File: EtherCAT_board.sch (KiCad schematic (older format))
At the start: 28 parts, among them J1 CONN_01X12, J2 USB_OTG, J3 RJ45-PULSETRANS, J4 RJ45-PULSETRANS, SW1 SKRPACE010, U1 LAN9252, U2 LM1117-3.3

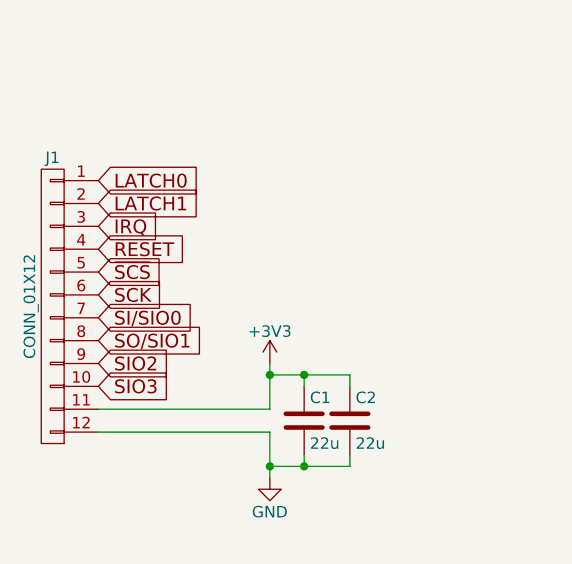
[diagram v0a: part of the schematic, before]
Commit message: 進捗
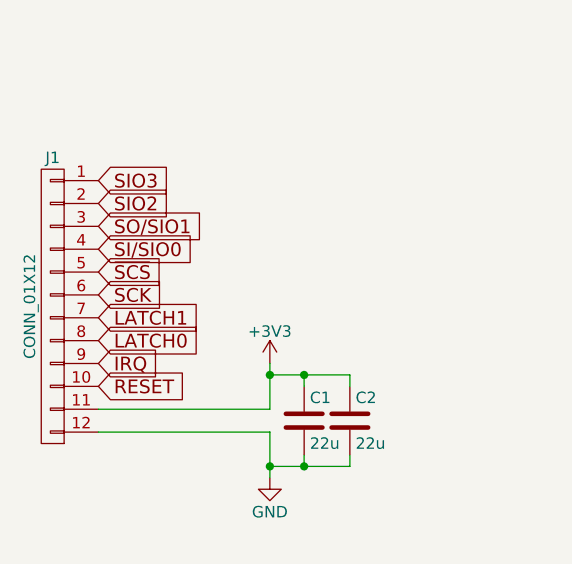
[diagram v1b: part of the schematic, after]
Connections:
- net IRQ: now also J1.9 (P9); no longer J1.3 (P3)
- net LATCH0: now also J1.8 (P8); no longer J1.1 (P1)
- net LATCH1: now also J1.7 (P7); no longer J1.2 (P2)
- net RESET: now also J1.10 (P10); no longer J1.4 (P4)
- net SI/SIO0: now also J1.4 (P4); no longer J1.7 (P7)
- net SIO2: now also J1.2 (P2); no longer J1.9 (P9)
- net SIO3: now also J1.1 (P1); no longer J1.10 (P10)
- net SO/SIO1: now also J1.3 (P3); no longer J1.8 (P8)
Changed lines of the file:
@@
 $EndComp
 $Comp
-L +3V3 #PWR17
+L +3V3 #PWR01
 U 1 1 5922F51B
 P 8850 4700
-F 0 "#PWR17" H 8850 4550 50  0001 C CNN
+F 0 "#PWR01" H 8850 4550 50  0001 C CNN
 F 1 "+3V3" H 8850 4840 50  0000 C CNN
 F 2 "" H 8850 4700 50  0001 C CNN
@@
 $EndComp
 $Comp
-L +3V3 #PWR16
+L +3V3 #PWR02
 U 1 1 5922FF45
 P 8850 2800
-F 0 "#PWR16" H 8850 2650 50  0001 C CNN
+F 0 "#PWR02" H 8850 2650 50  0001 C CNN
 F 1 "+3V3" H 8850 2940 50  0000 C CNN
 F 2 "" H 8850 2800 50  0001 C CNN
@@
 $EndComp
 $Comp
-L GND #PWR19
+L GND #PWR03
 U 1 1 5922FEB9
 P 10300 4350
-F 0 "#PWR19" H 10300 4100 50  0001 C CNN
+F 0 "#PWR03" H 10300 4100 50  0001 C CNN
 F 1 "GND" H 10300 4200 50  0000 C CNN
 F 2 "" H 10300 4350 50  0001 C CNN
@@
 $EndComp
 $Comp
-L GNDPWR #PWR21
+L GNDPWR #PWR04
 U 1 1 5922FF05
 P 10700 4350
-F 0 "#PWR21" H 10700 4150 50  0001 C CNN
+F 0 "#PWR04" H 10700 4150 50  0001 C CNN
 F 1 "GNDPWR" H 10700 4220 50  0000 C CNN
 F 2 "" H 10700 4300 50  0001 C CNN
@@
 $EndComp
 $Comp
-L GNDPWR #PWR22
+L GNDPWR #PWR05
 U 1 1 5923028E
 P 10700 6250
-F 0 "#PWR22" H 10700 6050 50  0001 C CNN
+F 0 "#PWR05" H 10700 6050 50  0001 C CNN
 F 1 "GNDPWR" H 10700 6120 50  0000 C CNN
 F 2 "" H 10700 6200 50  0001 C CNN
@@
 $EndComp
 $Comp
-L GND #PWR20
+L GND #PWR06
 U 1 1 5923041F
 P 10300 6250
-F 0 "#PWR20" H 10300 6000 50  0001 C CNN
+F 0 "#PWR06" H 10300 6000 50  0001 C CNN
 F 1 "GND" H 10300 6100 50  0000 C CNN
 F 2 "" H 10300 6250 50  0001 C CNN
@@
 $EndComp
 $Comp
-L GNDPWR #PWR23
+L GNDPWR #PWR07
 U 1 1 592307DA
 P 10950 4100
-F 0 "#PWR23" H 10950 3900 50  0001 C CNN
+F 0 "#PWR07" H 10950 3900 50  0001 C CNN
 F 1 "GNDPWR" H 10950 3970 50  0000 C CNN
 F 2 "" H 10950 4050 50  0001 C CNN
@@
 $EndComp
 $Comp
-L GNDPWR #PWR24
+L GNDPWR #PWR08
 U 1 1 5923094F
 P 10950 6000
-F 0 "#PWR24" H 10950 5800 50  0001 C CNN
+F 0 "#PWR08" H 10950 5800 50  0001 C CNN
 F 1 "GNDPWR" H 10950 5870 50  0000 C CNN
 F 2 "" H 10950 5950 50  0001 C CNN
@@
 $EndComp
 $Comp
-L GND #PWR14
+L GND #PWR09
 U 1 1 592A4371
 P 8600 4000
-F 0 "#PWR14" H 8600 3750 50  0001 C CNN
+F 0 "#PWR09" H 8600 3750 50  0001 C CNN
 F 1 "GND" H 8600 3850 50  0000 C CNN
 F 2 "" H 8600 4000 50  0001 C CNN
@@
 $EndComp
 $Comp
-L GND #PWR15
+L GND #PWR010
 U 1 1 592A4F5E
 P 8600 5900
-F 0 "#PWR15" H 8600 5650 50  0001 C CNN
+F 0 "#PWR010" H 8600 5650 50  0001 C CNN
 F 1 "GND" H 8600 5750 50  0000 C CNN
 F 2 "" H 8600 5900 50  0001 C CNN
@@
 $EndComp
 $Comp
-L +3V3 #PWR10
+L +3V3 #PWR011
 U 1 1 592B3DAC
 P 6550 2550
-F 0 "#PWR10" H 6550 2400 50  0001 C CNN
+F 0 "#PWR011" H 6550 2400 50  0001 C CNN
 F 1 "+3V3" H 6550 2690 50  0000 C CNN
 F 2 "" H 6550 2550 50  0001 C CNN
@@
 $EndComp
 $Comp
-L GND #PWR11
+L GND #PWR012
 U 1 1 592B401A
 P 6550 3350
-F 0 "#PWR11" H 6550 3100 50  0001 C CNN
+F 0 "#PWR012" H 6550 3100 50  0001 C CNN
 F 1 "GND" H 6550 3200 50  0000 C CNN
 F 2 "" H 6550 3350 50  0001 C CNN
@@
 $EndComp
 $Comp
-L GND #PWR3
+L GND #PWR013
 U 1 1 59240EF6
 P 5050 1750
-F 0 "#PWR3" H 5050 1500 50  0001 C CNN
+F 0 "#PWR013" H 5050 1500 50  0001 C CNN
 F 1 "GND" H 5050 1600 50  0000 C CNN
 F 2 "" H 5050 1750 50  0001 C CNN
@@
 $EndComp
 $Comp
-L GND #PWR4
+L GND #PWR014
 U 1 1 59242075
 P 5150 1750
-F 0 "#PWR4" H 5150 1500 50  0001 C CNN
+F 0 "#PWR014" H 5150 1500 50  0001 C CNN
 F 1 "GND" H 5150 1600 50  0000 C CNN
 F 2 "" H 5150 1750 50  0001 C CNN
@@
 NoConn ~ 5650 3150
 $Comp
-L GND #PWR8
+L GND #PWR015
 U 1 1 592521B8
 P 6150 3350
-F 0 "#PWR8" H 6150 3100 50  0001 C CNN
+F 0 "#PWR015" H 6150 3100 50  0001 C CNN
 F 1 "GND" H 6150 3200 50  0000 C CNN
 F 2 "" H 6150 3350 50  0001 C CNN
@@
 IRQ
 $Comp
-L +3V3 #PWR5
+L +3V3 #PWR016
 U 1 1 5927681F
 P 5450 3850
-F 0 "#PWR5" H 5450 3700 50  0001 C CNN
+F 0 "#PWR016" H 5450 3700 50  0001 C CNN
 F 1 "+3V3" H 5450 3990 50  0000 C CNN
 F 2 "" H 5450 3850 50  0001 C CNN
@@
 $EndComp
 $Comp
-L GND #PWR6
+L GND #PWR017
 U 1 1 59277FBB
 P 5450 4450
-F 0 "#PWR6" H 5450 4200 50  0001 C CNN
+F 0 "#PWR017" H 5450 4200 50  0001 C CNN
 F 1 "GND" H 5450 4300 50  0000 C CNN
 F 2 "" H 5450 4450 50  0001 C CNN
@@
 	-1   0    0    -1
 $EndComp
-Text GLabel 2250 5900 2    60   Input ~ 0
+Text GLabel 2250 6400 2    60   Input ~ 0
 LATCH1
-Text GLabel 2250 5800 2    60   Input ~ 0
+Text GLabel 2250 6500 2    60   Input ~ 0
 LATCH0
-Text GLabel 2250 6000 2    60   Input ~ 0
+Text GLabel 2250 6600 2    60   Input ~ 0
 IRQ
-Text GLabel 2250 6100 2    60   Input ~ 0
+Text GLabel 2250 6700 2    60   Input ~ 0
 RESET
 Text GLabel 2250 6200 2    60   Input ~ 0
@@
 Text GLabel 2250 6300 2    60   Input ~ 0
 SCK
-Text GLabel 2250 6400 2    60   Input ~ 0
+Text GLabel 2250 6100 2    60   Input ~ 0
 SI/SIO0
-Text GLabel 2250 6500 2    60   Input ~ 0
+Text GLabel 2250 6000 2    60   Input ~ 0
 SO/SIO1
-Text GLabel 2250 6600 2    60   Input ~ 0
+Text GLabel 2250 5900 2    60   Input ~ 0
 SIO2
-Text GLabel 2250 6700 2    60   Input ~ 0
+Text GLabel 2250 5800 2    60   Input ~ 0
 SIO3
 $Comp
-L +3V3 #PWR1
+L +3V3 #PWR018
 U 1 1 5928CFF9
 P 3000 6600
-F 0 "#PWR1" H 3000 6450 50  0001 C CNN
+F 0 "#PWR018" H 3000 6450 50  0001 C CNN
 F 1 "+3V3" H 3000 6740 50  0000 C CNN
 F 2 "" H 3000 6600 50  0001 C CNN
@@
 $EndComp
 $Comp
-L GND #PWR2
+L GND #PWR019
 U 1 1 5928E4C7
 P 3000 7100
-F 0 "#PWR2" H 3000 6850 50  0001 C CNN
+F 0 "#PWR019" H 3000 6850 50  0001 C CNN
 F 1 "GND" H 3000 6950 50  0000 C CNN
 F 2 "" H 3000 7100 50  0001 C CNN
@@
 $EndComp
 $Comp
-L +5V #PWR9
+L +5V #PWR020
 U 1 1 592C88B8
 P 6250 1000
-F 0 "#PWR9" H 6250 850 50  0001 C CNN
+F 0 "#PWR020" H 6250 850 50  0001 C CNN
 F 1 "+5V" H 6250 1140 50  0000 C CNN
 F 2 "" H 6250 1000 50  0001 C CNN
@@
 $EndComp
 $Comp
-L +3V3 #PWR13
+L +3V3 #PWR021
 U 1 1 592C980E
 P 7100 1000
-F 0 "#PWR13" H 7100 850 50  0001 C CNN
+F 0 "#PWR021" H 7100 850 50  0001 C CNN
 F 1 "+3V3" H 7100 1140 50  0000 C CNN
 F 2 "" H 7100 1000 50  0001 C CNN
@@
 Connection ~ 6700 1600
 $Comp
-L GND #PWR12
+L GND #PWR022
 U 1 1 592CCB1A
 P 6700 1700
-F 0 "#PWR12" H 6700 1450 50  0001 C CNN
+F 0 "#PWR022" H 6700 1450 50  0001 C CNN
 F 1 "GND" H 6700 1550 50  0000 C CNN
 F 2 "" H 6700 1700 50  0001 C CNN
@@
 	5850 1150 6400 1150
 $Comp
-L PWR_FLAG #FLG3
+L PWR_FLAG #FLG023
 U 1 1 592D234F
 P 7550 1000
-F 0 "#FLG3" H 7550 1075 50  0001 C CNN
+F 0 "#FLG023" H 7550 1075 50  0001 C CNN
 F 1 "PWR_FLAG" H 7550 1150 50  0000 C CNN
 F 2 "" H 7550 1000 50  0001 C CNN
@@
 	7550 1150 7550 1000
 $Comp
-L PWR_FLAG #FLG4
+L PWR_FLAG #FLG024
 U 1 1 592D2BA7
 P 7550 1450
-F 0 "#FLG4" H 7550 1525 50  0001 C CNN
+F 0 "#FLG024" H 7550 1525 50  0001 C CNN
 F 1 "PWR_FLAG" H 7550 1600 50  0000 C CNN
 F 2 "" H 7550 1450 50  0001 C CNN
@@
 Connection ~ 7100 1600
 $Comp
-L GNDPWR #PWR18
+L GNDPWR #PWR025
 U 1 1 592D7825
 P 9750 4500
-F 0 "#PWR18" H 9750 4300 50  0001 C CNN
+F 0 "#PWR025" H 9750 4300 50  0001 C CNN
 F 1 "GNDPWR" H 9750 4370 50  0000 C CNN
 F 2 "" H 9750 4450 50  0001 C CNN
@@
 $EndComp
 $Comp
-L PWR_FLAG #FLG5
+L PWR_FLAG #FLG026
 U 1 1 592D7B3F
 P 9750 4500
-F 0 "#FLG5" H 9750 4575 50  0001 C CNN
+F 0 "#FLG026" H 9750 4575 50  0001 C CNN
 F 1 "PWR_FLAG" H 9750 4650 50  0000 C CNN
 F 2 "" H 9750 4500 50  0001 C CNN
@@
 $EndComp
 $Comp
-L PWR_FLAG #FLG2
+L PWR_FLAG #FLG027
 U 1 1 592D7C8B
 P 5950 1000
-F 0 "#FLG2" H 5950 1075 50  0001 C CNN
+F 0 "#FLG027" H 5950 1075 50  0001 C CNN
 F 1 "PWR_FLAG" H 5950 1150 50  0000 C CNN
 F 2 "" H 5950 1000 50  0001 C CNN
@@
 Connection ~ 5950 1150
 $Comp
-L PWR_FLAG #FLG1
+L PWR_FLAG #FLG028
 U 1 1 592D8703
 P 5500 1000
-F 0 "#FLG1" H 5500 1075 50  0001 C CNN
+F 0 "#FLG028" H 5500 1075 50  0001 C CNN
 F 1 "PWR_FLAG" H 5500 1150 50  0000 C CNN
 F 2 "" H 5500 1000 50  0001 C CNN
@@
 Connection ~ 5500 1150
 $Comp
-L GND #PWR7
+L GND #PWR029
 U 1 1 592B099F
 P 5950 1800
-F 0 "#PWR7" H 5950 1550 50  0001 C CNN
+F 0 "#PWR029" H 5950 1550 50  0001 C CNN
 F 1 "GND" H 5950 1650 50  0000 C CNN
 F 2 "" H 5950 1800 50  0001 C CNN
